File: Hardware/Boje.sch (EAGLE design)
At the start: 10 parts, among them IC1 TINY13V-10PU, J1 332-02, J2 332-02

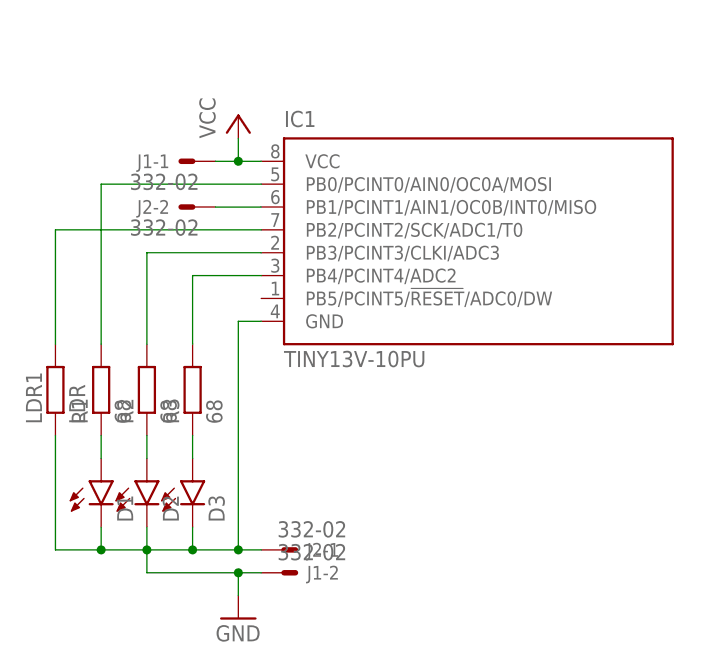
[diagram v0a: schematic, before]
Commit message: Board Update
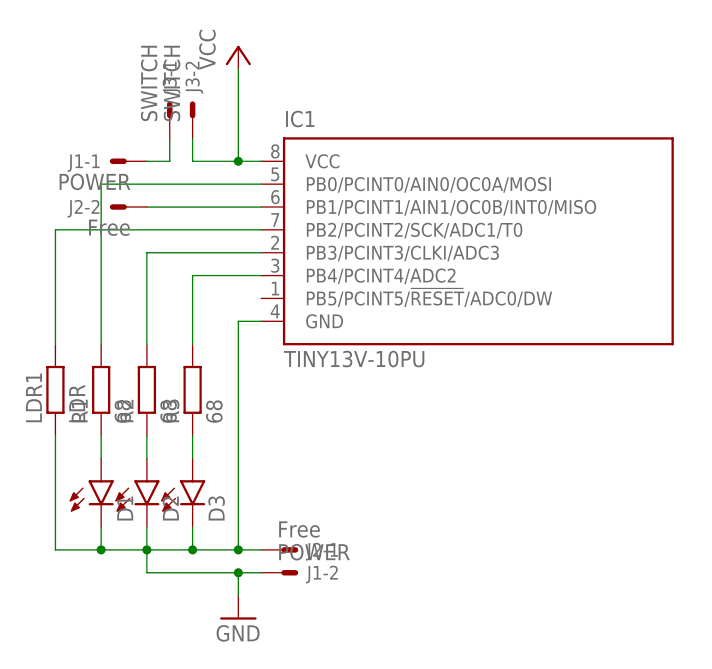
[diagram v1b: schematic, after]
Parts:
- added J3: SWITCH, con-garry:332-02
- J1: value 332-02 -> POWER
- J2: value 332-02 -> Free
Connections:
- new net N$1: J1-1.S, J3-1.S
- net VCC-5V: now also J3-2.S; no longer J1-1.S
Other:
- moved on the sheet: J1-1, J2-2
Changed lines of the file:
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@@
 <part name="R1" library="resistor" deviceset="R-EU_" device="M2012" value="68"/>
 <part name="LDR1" library="rcl" deviceset="R-EU_" device="V526-0" value="LDR"/>
-<part name="J1" library="con-garry" deviceset="332-02" device=""/>
-<part name="J2" library="con-garry" deviceset="332-02" device=""/>
+<part name="J1" library="con-garry" deviceset="332-02" device="" value="POWER"/>
+<part name="J2" library="con-garry" deviceset="332-02" device="" value="Free"/>
+<part name="J3" library="con-garry" deviceset="332-02" device="" value="SWITCH"/>
 </parts>
 <sheets>
@@
 <instances>
 <instance part="IC1" gate="G$1" x="45.72" y="38.1"/>
-<instance part="P+2" gate="VCC" x="22.86" y="55.88"/>
+<instance part="P+2" gate="VCC" x="22.86" y="63.5"/>
 <instance part="GND8" gate="1" x="22.86" y="0"/>
 <instance part="D3" gate="G$1" x="17.78" y="15.24"/>
@@
 <instance part="R1" gate="G$1" x="7.62" y="25.4" rot="R90"/>
 <instance part="LDR1" gate="G$1" x="2.54" y="25.4" rot="R90"/>
-<instance part="J1" gate="-1" x="17.78" y="50.8" rot="R180"/>
+<instance part="J1" gate="-1" x="10.16" y="50.8" rot="R180"/>
 <instance part="J1" gate="-2" x="27.94" y="5.08"/>
 <instance part="J2" gate="-1" x="27.94" y="7.62"/>
-<instance part="J2" gate="-2" x="17.78" y="45.72" rot="R180"/>
+<instance part="J2" gate="-2" x="10.16" y="45.72" rot="R180"/>
+<instance part="J3" gate="-1" x="15.24" y="55.88" rot="R90"/>
+<instance part="J3" gate="-2" x="17.78" y="55.88" rot="R90"/>
 </instances>
 <busses>
@@
 <pinref part="P+2" gate="VCC" pin="VCC"/>
 <wire x1="25.4" y1="50.8" x2="22.86" y2="50.8" width="0.1524" layer="91"/>
-<wire x1="22.86" y1="50.8" x2="22.86" y2="53.34" width="0.1524" layer="91"/>
-<pinref part="J1" gate="-1" pin="S"/>
-<wire x1="22.86" y1="50.8" x2="20.32" y2="50.8" width="0.1524" layer="91"/>
+<wire x1="22.86" y1="50.8" x2="22.86" y2="60.96" width="0.1524" layer="91"/>
+<wire x1="22.86" y1="50.8" x2="17.78" y2="50.8" width="0.1524" layer="91"/>
 <junction x="22.86" y="50.8"/>
+<wire x1="17.78" y1="53.34" x2="17.78" y2="50.8" width="0.1524" layer="91"/>
+<pinref part="J3" gate="-2" pin="S"/>
 </segment>
 </net>
@@
 <pinref part="IC1" gate="G$1" pin="PB1/PCINT1/AIN1/OC0B/INT0/MISO"/>
 <pinref part="J2" gate="-2" pin="S"/>
-<wire x1="25.4" y1="45.72" x2="20.32" y2="45.72" width="0.1524" layer="91"/>
+<wire x1="25.4" y1="45.72" x2="12.7" y2="45.72" width="0.1524" layer="91"/>
 </segment>
 </net>
+<net name="N$1" class="0">
+<segment>
+<pinref part="J1" gate="-1" pin="S"/>
+<pinref part="J3" gate="-1" pin="S"/>
+<wire x1="15.24" y1="50.8" x2="15.24" y2="53.34" width="0.1524" layer="91"/>
+<wire x1="15.24" y1="50.8" x2="12.7" y2="50.8" width="0.1524" layer="91"/>
+</segment>
+</net>
